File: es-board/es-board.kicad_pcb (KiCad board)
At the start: 2 copper layers, 81.4 x 42.1 mm, 54 parts, among them J1 Conn_02x02_Odd_Even, J3 USB_C_Receptacle_USB2.0, Q1 Q_PMOS_GSD, Q2 Q_PMOS_GSD, Q3 Q_PMOS_GSD, Q4 Q_PMOS_GSD, Q5 NMOS, SW1 SW_SPST, SW2 SW_SPST, SW3 SW_SPST, SW4 SW_SPST, SW5 SW_SPST, U1 CYPD3177, U2 ATmega32U4-A, U3 IP4234CZ6,125, U4 IFX25001TFV50ATMA1, U5 OLED, Y1 16MHz Crystal

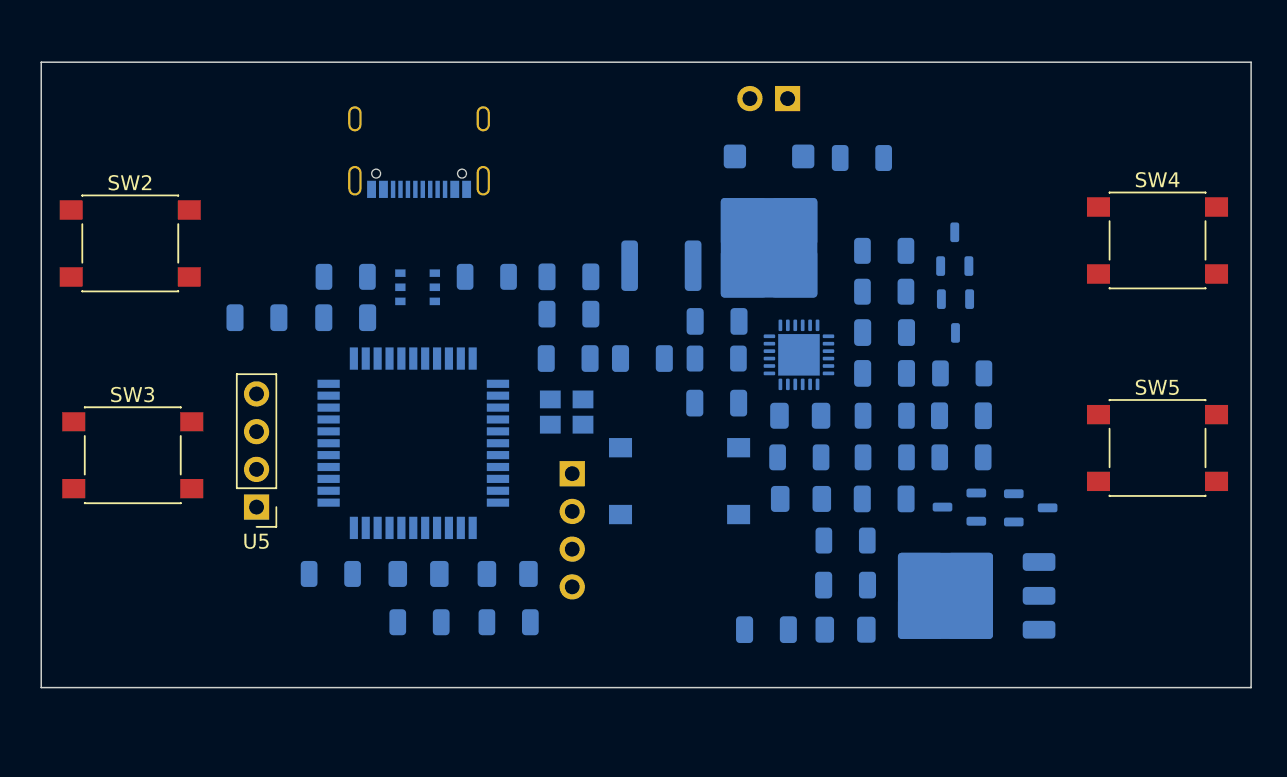
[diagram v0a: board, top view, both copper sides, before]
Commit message: Did some routing
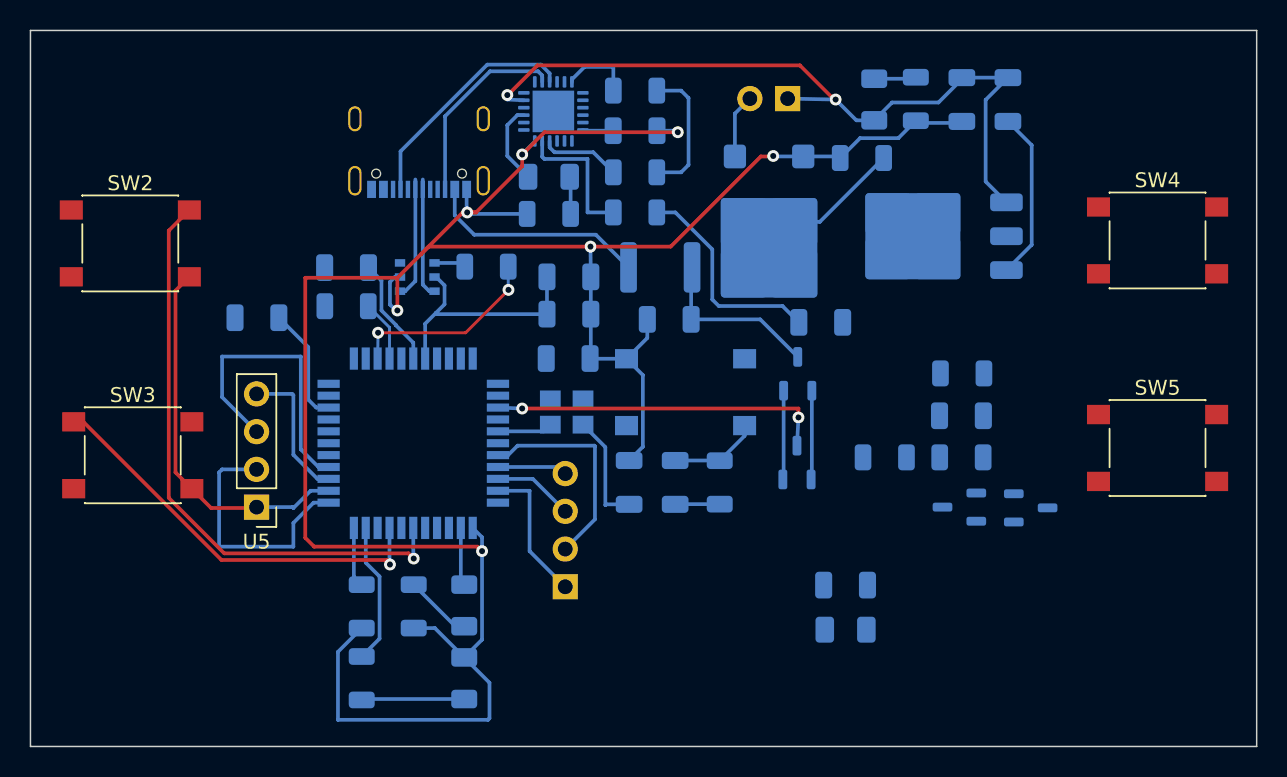
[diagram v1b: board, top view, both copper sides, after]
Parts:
- moved C13 39.2 mm to (170.7, 69.5), turned to -90 degrees
- moved R4 29.7 mm to (139.8, 77.2), turned to 180 degrees
- moved D3 27.5 mm to (139.8, 74.7)
- moved C10 27.4 mm to (167.6, 69.5), turned to -90 degrees
- moved R13 25.4 mm to (164.5, 69.5), turned to -90 degrees
- moved U4 24.3 mm to (165.6, 78.7)
- moved C11 23.4 mm to (145.6, 71.6), turned to 0 degrees
- moved U1 23.3 mm to (140.1, 70.3), turned to 90 degrees
- moved D4 21.9 mm to (161.7, 69.5), turned to -90 degrees
- moved R12 21.7 mm to (145.6, 77.1)
- moved R11 19.9 mm to (145.6, 68.9)
- moved R10 18.6 mm to (145.6, 74.4)
- moved Q4 14.5 mm to (156.5, 93.9), turned to 90 degrees
- moved Q3 13.5 mm to (156.6, 88.0)
- moved C2 8.39 mm to (145.2, 95.3), turned to 90 degrees
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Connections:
- SW2 pad 1: io8 - UP -> io8
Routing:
- net GND: track 0.00 -> 196.6 mm, vias 0 -> 7
- net +5V: track 0.00 -> 63.5 mm, vias 0 -> 2
- net VBUS: track 0.00 -> 51.4 mm, vias 0 -> 2
- net io8: track 0.00 -> 40.1 mm, vias 0 -> 1
- net io10: track 0.00 -> 27.8 mm, vias 0 -> 1
- net a1: track 0.00 -> 19.9 mm
- net Net-(Q1-D): track 0.00 -> 16.4 mm
- net USB_CC1: track 0.00 -> 15.8 mm
- net Net-(Q3-G): track 0.00 -> 15.2 mm
- net VBUS_RAW: track 0.00 -> 14.9 mm
- net /Power/3v3_usbpd: track 0.00 -> 14.6 mm
- net d3/scl: track 0.00 -> 14.6 mm
- net USB_D-: track 0.00 -> 13.3 mm, vias 0 -> 2
- net USB_CC2: track 0.00 -> 13.3 mm
- net Net-(D5-A): track 0.00 -> 11.4 mm
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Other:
- board size 81.4 x 42.1 mm -> 82.5 x 48.2 mm
